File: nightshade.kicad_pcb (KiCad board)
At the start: 4 copper layers, 153.3 x 70.8 mm, 81 parts, among them J1 Bus_ISA_16bit, J2 DE15_Plug_HighDensity_Mountin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, U1 GD542x_ISA, U2 SOJ_256Kx16, U3 SOJ_256Kx16, U4 LM334M, U5 LDK320AM50R, U6 27C256, U7 74LS244, Y1 14.31818MHz

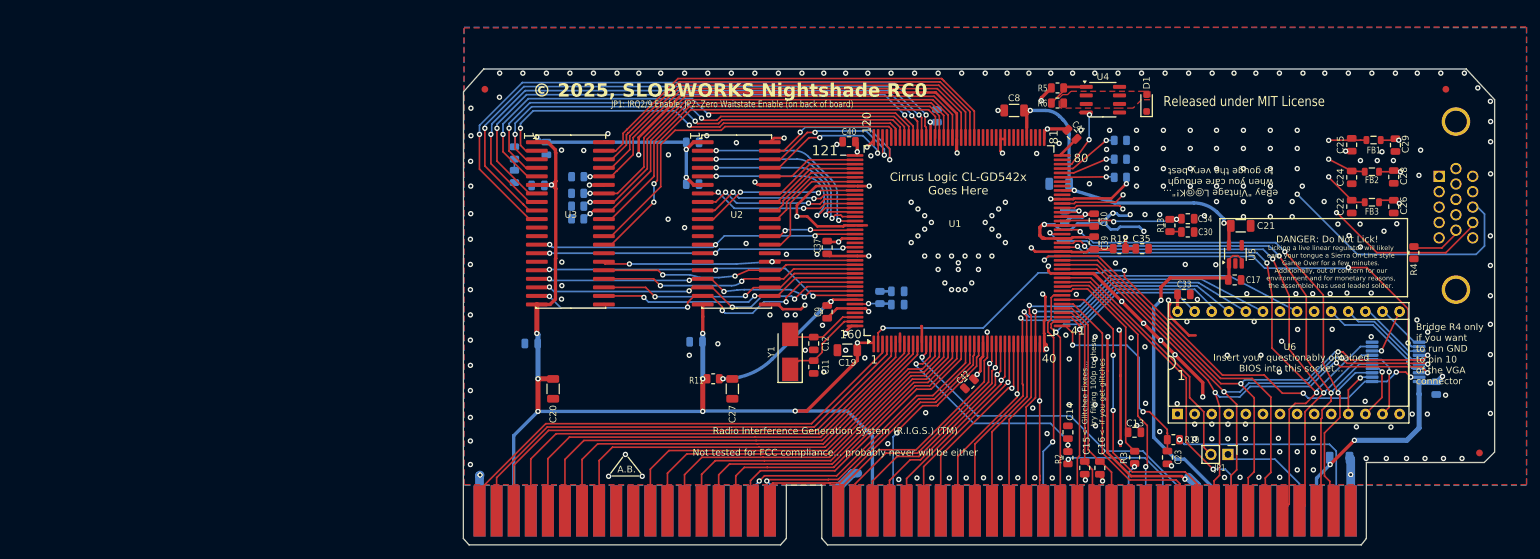
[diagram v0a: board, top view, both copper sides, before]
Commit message: Add files via upload
Updated to Cherry Tomato V1.0 revision
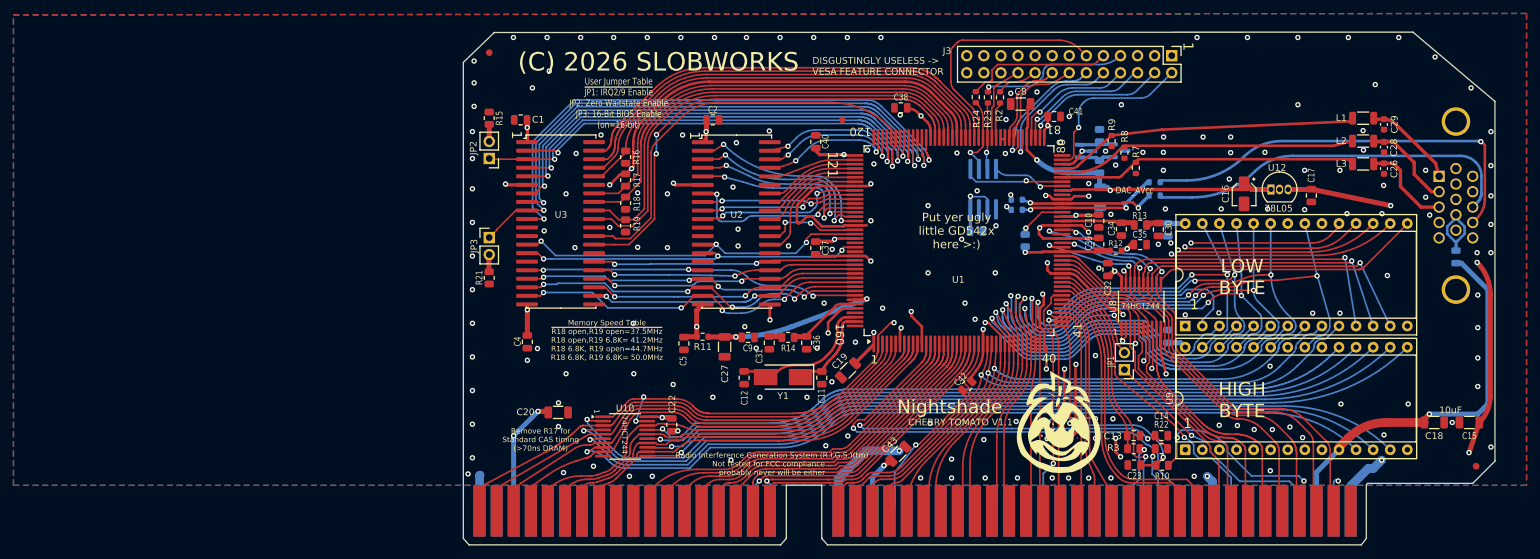
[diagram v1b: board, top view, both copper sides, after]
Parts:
- removed C21: 10u, Capacitor_SMD:C_1206_3216Metric
- removed C3, C6: 0.22u, Capacitor_SMD:C_0805_2012Metric
- removed D1: 1N4148WS, Diode_SMD:D_SOD-323_HandSoldering
- removed FB1, FB2, FB3: 0805, Inductor_SMD:L_0805_2012Metric
- removed the G*** at (127.9, 117.0)
- removed U7: 74LS244, Package_SO:SSOP-20_5.3x7.2mm_P0.65mm
- added C43: 10u, Capacitor_SMD:C_1206_3216Metric, F.Cu at (145.6, 144.4)
- added F1: 0805L020YR, Fuse:Fuse_0805_2012Metric, B.Cu at (228.5, 115.1)
- added G***: LOGO, SOJ_DRAM:tomato2, F.Cu at (169.5, 139.8)
- added J3: Conn_02x13_Odd_Even, Connector_PinHeader_2.54mm:PinHeader_2x13_P2.54mm_Vertical, F.Cu at (186.2, 85.2)
- added JP3: 16bit_BIOS, Connector_PinHeader_2.54mm:PinHeader_1x02_P2.54mm_Vertical, F.Cu at (84.8, 112.2)
- added L1: 1210, Inductor_SMD:L_1206_3216Metric, F.Cu at (214.7, 94.5)
- added L2: 1210, Inductor_SMD:L_1206_3216Metric, F.Cu at (214.7, 97.9)
- added L3: 1210, Inductor_SMD:L_1206_3216Metric, F.Cu at (214.7, 101.3)
- added Q1: MMBT3904, Package_TO_SOT_SMD:SOT-23, B.Cu at (173.5, 99.4)
- added R20: 33, Resistor_SMD:R_0603_1608Metric, B.Cu at (163.2, 108.1)
- added R21: 6.8K, Resistor_SMD:R_0805_2012Metric, F.Cu at (84.8, 118.2)
- added R22: 33, Resistor_SMD:R_0805_2012Metric, F.Cu at (184.7, 143.7)
- added R23: 1K, Resistor_SMD:R_0603_1608Metric, F.Cu at (158.9, 91.4)
- added R24: 1K, Resistor_SMD:R_0603_1608Metric, F.Cu at (157.1, 91.4)
- added R25: 16, Resistor_SMD:R_0603_1608Metric, B.Cu at (183.7, 104.0)
- added R26: 16, Resistor_SMD:R_0603_1608Metric, B.Cu at (183.7, 106.0)
- added U10: 74HCT244, PDVGA:SSOP-20_4.4_5.3x6.5mm_P0.65mm, F.Cu at (105.0, 141.8)
- added U12: L78L05_TO92, Package_TO_SOT_THT:TO-92_Inline, F.Cu at (201.0, 105.1)
- added U8: 74HCT244, PDVGA:SSOP-20_4.4_5.3x6.5mm_P0.65mm, F.Cu at (181.7, 122.5)
- added U9: 27C256, Package_DIP:DIP-28_W15.24mm_Socket, F.Cu at (188.2, 143.8)
- C1, C2, C32, C36, C38, C4, C5: value 0.22u -> 0.1u; moved to F.Cu
- C10, C17, C34, C35, C37, C39, C40, C41, C42, C9: value 0.22u -> 0.1u
- C15: value 100p -> 10u; footprint Capacitor_SMD:C_0805_2012Metric -> Capacitor_SMD:C_1206_3216Metric
- C16: value 100p -> 4.7u; footprint Capacitor_SMD:C_0805_2012Metric -> Capacitor_SMD:CP_Elec_3x5.4
- C18, C31, R14, R15, R16, R17, R18, R19: moved to F.Cu
- C22: value 12p -> 0.1u
- C24, C25: value 12p -> 0.1u; moved to B.Cu
- C26, C28, C29: value 12p -> 47pF; footprint Capacitor_SMD:C_0805_2012Metric -> Capacitor_SMD:C_0603_1608Metric
- C33: value 0.22u -> 0.1u; moved to B.Cu
- C7, C8: value 2.2u -> 10u
- JP2: footprint Resistor_SMD:R_0805_2012Metric -> Connector_PinHeader_2.54mm:PinHeader_1x02_P2.54mm_Vertical; moved to F.Cu
- R11, R12: footprint Resistor_SMD:R_0805_2012Metric -> Resistor_SMD:R_0603_1608Metric
- R2: value 47 -> 33; footprint Resistor_SMD:R_0805_2012Metric -> Resistor_SMD:R_0603_1608Metric
- R4: value EhWot -> 33; footprint Resistor_SMD:R_0805_2012Metric -> Resistor_SMD:R_0603_1608Metric; moved to B.Cu
- R5: value 150 -> 1K; moved to B.Cu
- R6: value 15 -> 270-300; moved to B.Cu
- R7, R8, R9: footprint Resistor_SMD:R_0805_2012Metric -> Resistor_SMD:R_0603_1608Metric; moved to F.Cu
- U4: value LM334M -> TL431DBZ; footprint Package_SO:SOIC-8_3.9x4.9mm_P1.27mm -> Package_TO_SOT_SMD:SOT-23; moved to B.Cu
- U5: value LDK320AM50R -> 93CxxA; footprint Package_TO_SOT_SMD:SOT-23-5_HandSoldering -> PDVGA:SOIC-8_DMP-8; moved to B.Cu
- moved C22 106.2 mm to (111.9, 140.1)
- moved FID1 89.9 mm to (137.2, 94.8)
- moved R4 59.6 mm to (163.2, 106.6), turned to 180 degrees
- moved C15 57.6 mm to (230.5, 139.8), turned to 180 degrees
- moved C24 56.4 mm to (157.2, 111.3), turned to 180 degrees
- moved R2 54.5 mm to (160.7, 91.4)
- moved C32 51.9 mm to (176.8, 117.0), turned to -90 degrees
- moved C16 46.1 mm to (197.0, 105.8), turned to -90 degrees
- moved C25 39.5 mm to (185.7, 127.0), turned to -90 degrees
- moved U5 38.7 mm to (158.2, 105.0), turned to -90 degrees
- moved C5 23.7 mm to (113.7, 128.0), turned to 90 degrees
- moved C31 20.6 mm to (126.4, 127.9), turned to -90 degrees
- moved JP1 19.9 mm to (179.2, 131.9), turned to 180 degrees
- moved C17 17.0 mm to (207.0, 106.0), turned to -90 degrees
- moved C18 15.0 mm to (225.3, 139.8)
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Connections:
- net /~{MEMW} renamed /~{SMEMW}
- C15 pad 1: GND -> /+12V
- C15 pad 2: /SA15 -> GND
- C16 pad 1: GND -> /AVcc
- C16 pad 2: /SA16 -> GND
- C22 pad 2: /BLUE -> /+5V
- C24 pad 2: /GREEN -> /+5V
- C25 pad 2: /RED -> /+5V
- J1 pad 12: Net-(J1-~{SMEMR}) -> /~{SMEMR}
- J2 pad 10: Net-(J2-Pad10) -> GND
- J2 pad 13: /HSYNC -> /VHSYNC
- J2 pad 14: /VSYNC -> /VVSYNC
- J2 pad 9: unconnected-(J2-Pad9) -> Net-(F1-Pad2)
- R1 pad 2: /VCLKVCC -> /+5V
- R2 pad 1: Net-(J1-~{SMEMR}) -> /DCLK
- R2 pad 2: /~{MEMR} -> Net-(J3-Pin_18)
- R4 pad 1: Net-(J2-Pad10) -> /HSYNC
- R4 pad 2: GND -> /FHSYNC
- R5 pad 1: GND -> /AVcc
- R5 pad 2: Net-(R5-Pad2) -> Net-(Q1-B)
- R6 pad 1: Net-(R5-Pad2) -> Net-(Q1-E)
- R6 pad 2: Net-(D1-A) -> GND
- U1 pad 73: unconnected-(U1-EEDI-Pad73) -> /EEDI
- U1 pad 74: unconnected-(U1-EECS-Pad74) -> /EECS
- U4 pad 1: Net-(R5-Pad2) -> Net-(Q1-B)
- U4 pad 2: Net-(D1-A) -> Net-(Q1-E)
- U4 pad 3: Net-(D1-A) -> GND
- U5 pad 1: /+12V -> /EECS
- U5 pad 2: GND -> /ESYNC
- U5 pad 3: /+12V -> /EVIDEO
- U5 pad 4: unconnected-(U5-BP-Pad4) -> /EEDI
- U5 pad 5: /AVcc -> GND
- U6 pad 1: unconnected-(U6-VPP-Pad1) -> /+5V
- U6 pad 11: Net-(U6-D0) -> /D0
- U6 pad 12: Net-(U6-D1) -> /D1
- U6 pad 13: Net-(U6-D2) -> /D2
- U6 pad 15: Net-(U6-D3) -> /D3
- U6 pad 16: Net-(U6-D4) -> /D4
- U6 pad 17: Net-(U6-D5) -> /D5
- U6 pad 18: Net-(U6-D6) -> /D6
- U6 pad 19: Net-(U6-D7) -> /D7
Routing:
- net /+5V: track 457.5 -> 207.3 mm, vias 21 -> 20
- net /D11: track 0.00 -> 132.1 mm, vias 0 -> 1
- net /D10: track 0.00 -> 129.2 mm, vias 0 -> 1
- net /D9: track 0.00 -> 124.5 mm, vias 0 -> 1
- net /D8: track 0.00 -> 122.4 mm, vias 0 -> 1
- net /D12: track 0.00 -> 115.5 mm, vias 0 -> 1
- net /D13: track 0.00 -> 112.5 mm, vias 0 -> 1
- net /D14: track 0.00 -> 109.5 mm, vias 0 -> 1
- net /D15: track 0.00 -> 108.0 mm, vias 0 -> 1
- net /SD3: track 124.3 -> 54.5 mm, vias 3 -> 0
- net GND: track 310.4 -> 242.6 mm, vias 310 -> 204
- net /VVSYNC: track 0.00 -> 62.1 mm, vias 0 -> 1
- net /VHSYNC: track 0.00 -> 56.2 mm
- net /+12V: track 55.0 -> 109.3 mm, vias 1 -> 4
- net /HSYNC: track 74.7 -> 20.5 mm
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- added copper zone on In2.Cu, net /+5V
- removed copper zone on F.Cu, net Net-(D1-A)
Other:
- board size 153.3 x 70.8 mm -> 153.4 x 76.2 mm
- board text added: "(C) 2026 SLOBWORKS"
- board text added: "(Optional)"
- board text added: "10uF"
- board text added: "27C256"
- board text added: "3904"
- board text added: "74HCT244"
- board text added: "78L05"
- board text added: "93C46"
- board text added: "C32"
- board text added: "CHERRY TOMATO V1.1"
- board text added: "DAC_AVcc"
- board text added: "DISGUSTINGLY USELESS -> VESA FEATURE CONNECTOR"
- board text added: "Designed by AB in California Released under MIT License"
- board text added: "HIGH BYTE"
- board text added: "LOW BYTE"
- board text added: "Memory Speed Table ~{R18 open,R19 open=37.5MHz} R18 open,R19 6.8K= 41.2MHz R18 6.8K, R19 open=44.7MHz R18 6.8K, R19 6.8K= 50.0MHz"
- board text added: "Nightshade"
- board text added: "Put yer ugly little GD542x here >:)"
- board text added: "Radio Interference Generation System (R.I.G.S.)(tm) Not tested for FCC compliance... probably never will be either"
- board text added: "THE 16-BIT STRAW OF PURE CHOKEHOLD"
- board text added: "TL431"
- board text added: "U6"
- board text added: "User Jumper Table ~{JP1: IRQ2/9 Enable} JP2: Zero Waitstate Enable JP3: 16-Bit BIOS Enable (on=16-bit)"
- board text added: "a27004a714f54ecec9eed07aae3e28bf"
- board text removed: "<- Glitchee Fixees... try fitting 100p to these, <- if you get glitches"
- board text removed: "A.B."
- board text removed: "Bridge R4 only if you want to run GND to pin 10 of the VGA connector"
- board text removed: "Cirrus Logic CL-GD542x Goes Here"
- board text removed: "DANGER: Do Not Lick!"
- board text removed: "Designed by AB in California"
- board text removed: "Insert your questionably obtained BIOS into this socket..."
- board text removed: "JP1: IRQ2/9 Enable, JP2: Zero Waitstate Enable (on back of board)"
- board text removed: "Licking a live linear regulator will likely earn your tongue a Sierra On-Line style Game Over for a few minutes. Additionally, out of concern for our environment and for monetary reasons, the assembler has used leaded solder."
- board text removed: "Memory Speed Table ------------- R18 open,R19 open=37.5MHz R18 open,R19 6.8K= 41.2MHz R18 6.8K, R19 open=44.7MHz R18 6.8K, R19 6.8K= 50.0MHz"
- board text removed: "Radio Interference Generation System (R.I.G.S.) (TM) Not tested for FCC compliance... probably never will be either"
- board text removed: "Released under MIT License"
- board text removed: "Unfortunately, circuit boards don't taste good. Do not ask me how I know"
- board text removed: "Who needs good"
- board text removed: "blue,"
- board text removed: "eBay "Vintage L@@K!"... when you care enough to gouge the very best"
- board text removed: "electrical layout"
- board text removed: "people?"
- board text removed: "puppy-dog"
- board text removed: "three-fingered"
- board text removed: "when we have"
- board text removed: "© 2025, SLOBWORKS Nightshade RC0"
